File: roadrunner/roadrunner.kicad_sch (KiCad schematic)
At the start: 84 parts, among them J1 Battery_conn, J2 battery_conn_r, J3 Conn_01x12_Female, J4 niceview_left, J5 niceview_right, J6 Conn_01x12_Female, SW1 SW_Push, SW10 SW_Push, SW10_r1 SW_Push, SW11 SW_Push, SW11_r1 SW_Push, SW12 SW_Push, SW12_r1 SW_Push, SW13 SW_Push, SW13_r1 SW_Push, SW14 SW_Push, SW14_r1 SW_Push, SW15 SW_Push, SW15_r1 SW_Push, SW16 SW_Push, SW16_r1 SW_Push, SW17 SW_Push, SW17_r1 SW_Push, SW1_r1 SW_Push, SW2 SW_Push, SW2_r1 SW_Push, SW3 SW_Push, SW3_r1 SW_Push, SW4 SW_Push, SW4_r1 SW_Push, SW5 SW_Push, SW5_r1 SW_Push, SW6 SW_Push, SW6_r1 SW_Push, SW7 SW_Push, SW7_r1 SW_Push, SW8 SW_Push, SW8_r1 SW_Push, SW9 SW_Push, SW9_r1 SW_Push, U1 ProMicro-kbd, U2 ProMicro-kbd

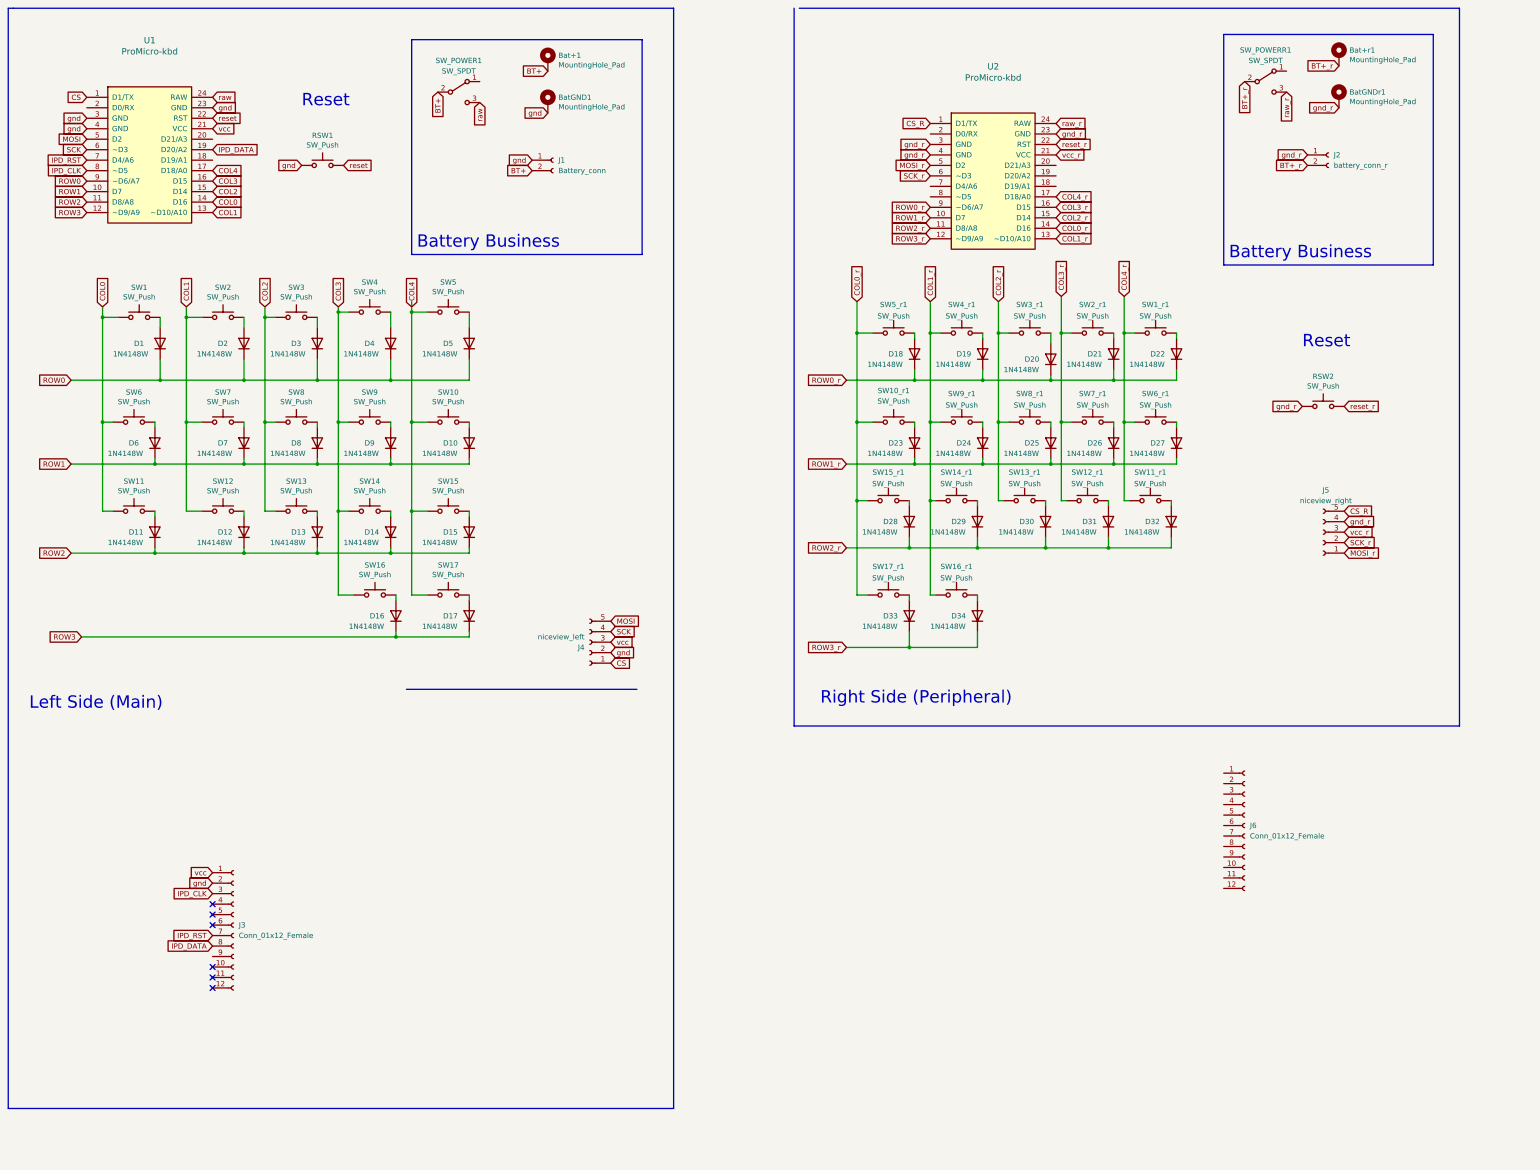
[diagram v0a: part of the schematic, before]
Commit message: feat: add vik
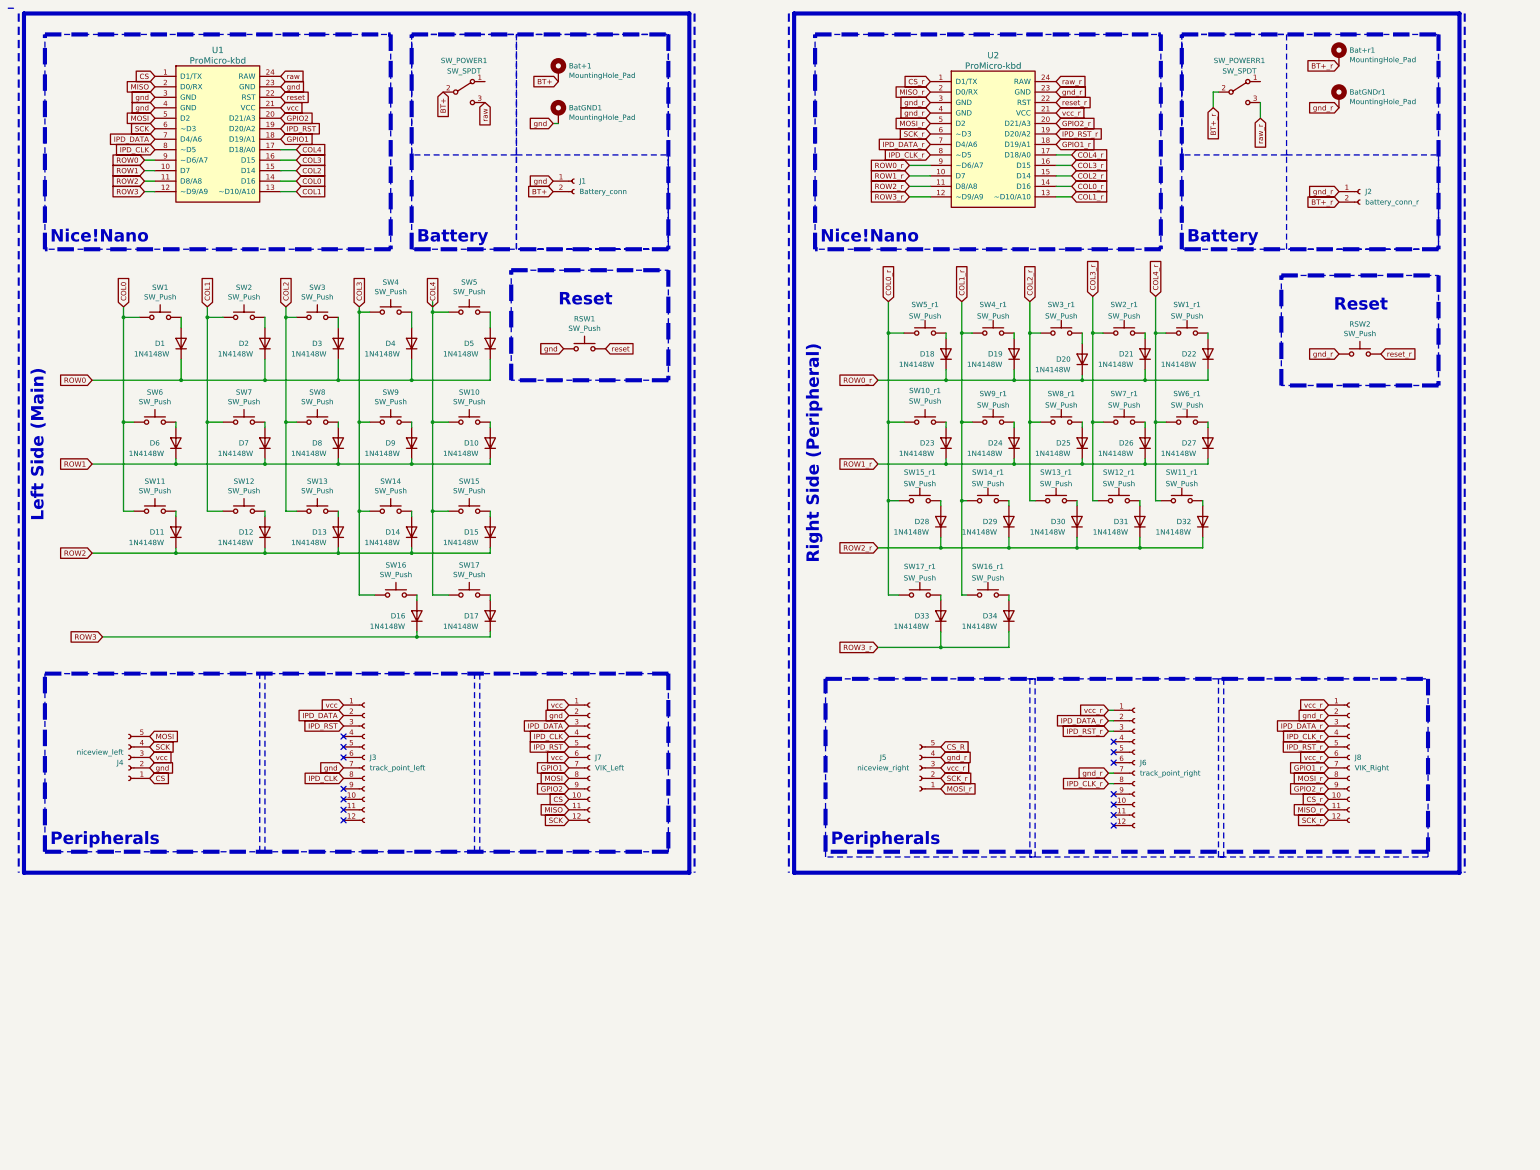
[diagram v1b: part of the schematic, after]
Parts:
- added J7: VIK_Left, Connector_FFC-FPC:Hirose_FH12-12S-0.5SH_1x12-1MP_P0.50mm_Horizontal, symbol Connector:Conn_01x12_Socket
- added J8: VIK_Right, Connector_FFC-FPC:Hirose_FH12-12S-0.5SH_1x12-1MP_P0.50mm_Horizontal, symbol Connector:Conn_01x12_Socket
- J3: value Conn_01x12_Female -> track_point_left; footprint Connector_FFC-FPC:Hirose_FH12-12S-0.5SH_1x12-1MP_P0.50mm_Horizontal -> Connector_FFC-FPC:TE_1-84953-2_1x12-1MP_P1.0mm_Horizontal
- J6: value Conn_01x12_Female -> track_point_right; footprint (none) -> Connector_FFC-FPC:TE_1-84953-2_1x12-1MP_P1.0mm_Horizontal
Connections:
- net CS: now also J7.10 (Pin_10)
- net CS_R: no longer U2.1 (D1/TX)
- net IPD_CLK: now also J3.8 (Pin_8), J7.4 (Pin_4); no longer J3.3 (Pin_3)
- net IPD_DATA: now also J3.2 (Pin_2), U1.7 (D4/A6), J7.3 (Pin_3); no longer J3.8 (Pin_8), U1.19 (D20/A2)
- net IPD_RST: now also J3.3 (Pin_3), U1.19 (D20/A2), J7.5 (Pin_5); no longer J3.7 (Pin_7), U1.7 (D4/A6)
- net MOSI: now also J7.8 (Pin_8)
- net MOSI_r: now also J8.8 (Pin_8)
- net SCK: now also J7.12 (Pin_12)
- net SCK_r: now also J8.12 (Pin_12)
- net gnd: now also J3.7 (Pin_7), J7.2 (Pin_2); no longer J3.2 (Pin_2)
- net gnd_r: now also J6.7 (Pin_7), J8.2 (Pin_2)
- net vcc: now also J7.1 (Pin_1), J7.6 (Pin_6)
- net vcc_r: now also J6.1 (Pin_1), J8.1 (Pin_1), J8.6 (Pin_6)
- net GPIO1_r: now reaches U2.18 (D19/A1)
- net GPIO1_r: now also J8.7 (Pin_7)
- net IPD_RST_r: now reaches U2.19 (D20/A2)
- net IPD_RST_r: now also J6.3 (Pin_3), J8.5 (Pin_5)
- net MISO_r: now reaches U2.2 (D0/RX)
- net MISO_r: now also J8.11 (Pin_11)
- net GPIO2_r: now reaches U2.20 (D21/A3)
- net GPIO2_r: now also J8.9 (Pin_9)
- net IPD_DATA_r: now reaches U2.7 (D4/A6)
- net IPD_DATA_r: now also J6.2 (Pin_2), J8.3 (Pin_3)
- net IPD_CLK_r: now reaches U2.8 (~D5)
- net IPD_CLK_r: now also J6.8 (Pin_8), J8.4 (Pin_4)
- net GPIO1: now reaches U1.18 (D19/A1)
- net GPIO1: now also J7.7 (Pin_7)
- net MISO: now reaches U1.2 (D0/RX)
- net MISO: now also J7.11 (Pin_11)
- net GPIO2: now reaches U1.20 (D21/A3)
- net GPIO2: now also J7.9 (Pin_9)
- new net CS_r: J8.10 (Pin_10), U2.1 (D1/TX)
- no-connect marks 6 -> 14
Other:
- note added: "Battery"
- note added: "Nice!Nano"
- note added: "Peripherals"
- note removed: "Battery Business"
- moved on the sheet: Bat+1, BatGND1, D1, D10, D11, D12, D13, D14, D15, D16, D17, D18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
